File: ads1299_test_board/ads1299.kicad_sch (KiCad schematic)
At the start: 30 parts, among them U1 ADS1299, U4 OPA376xxD

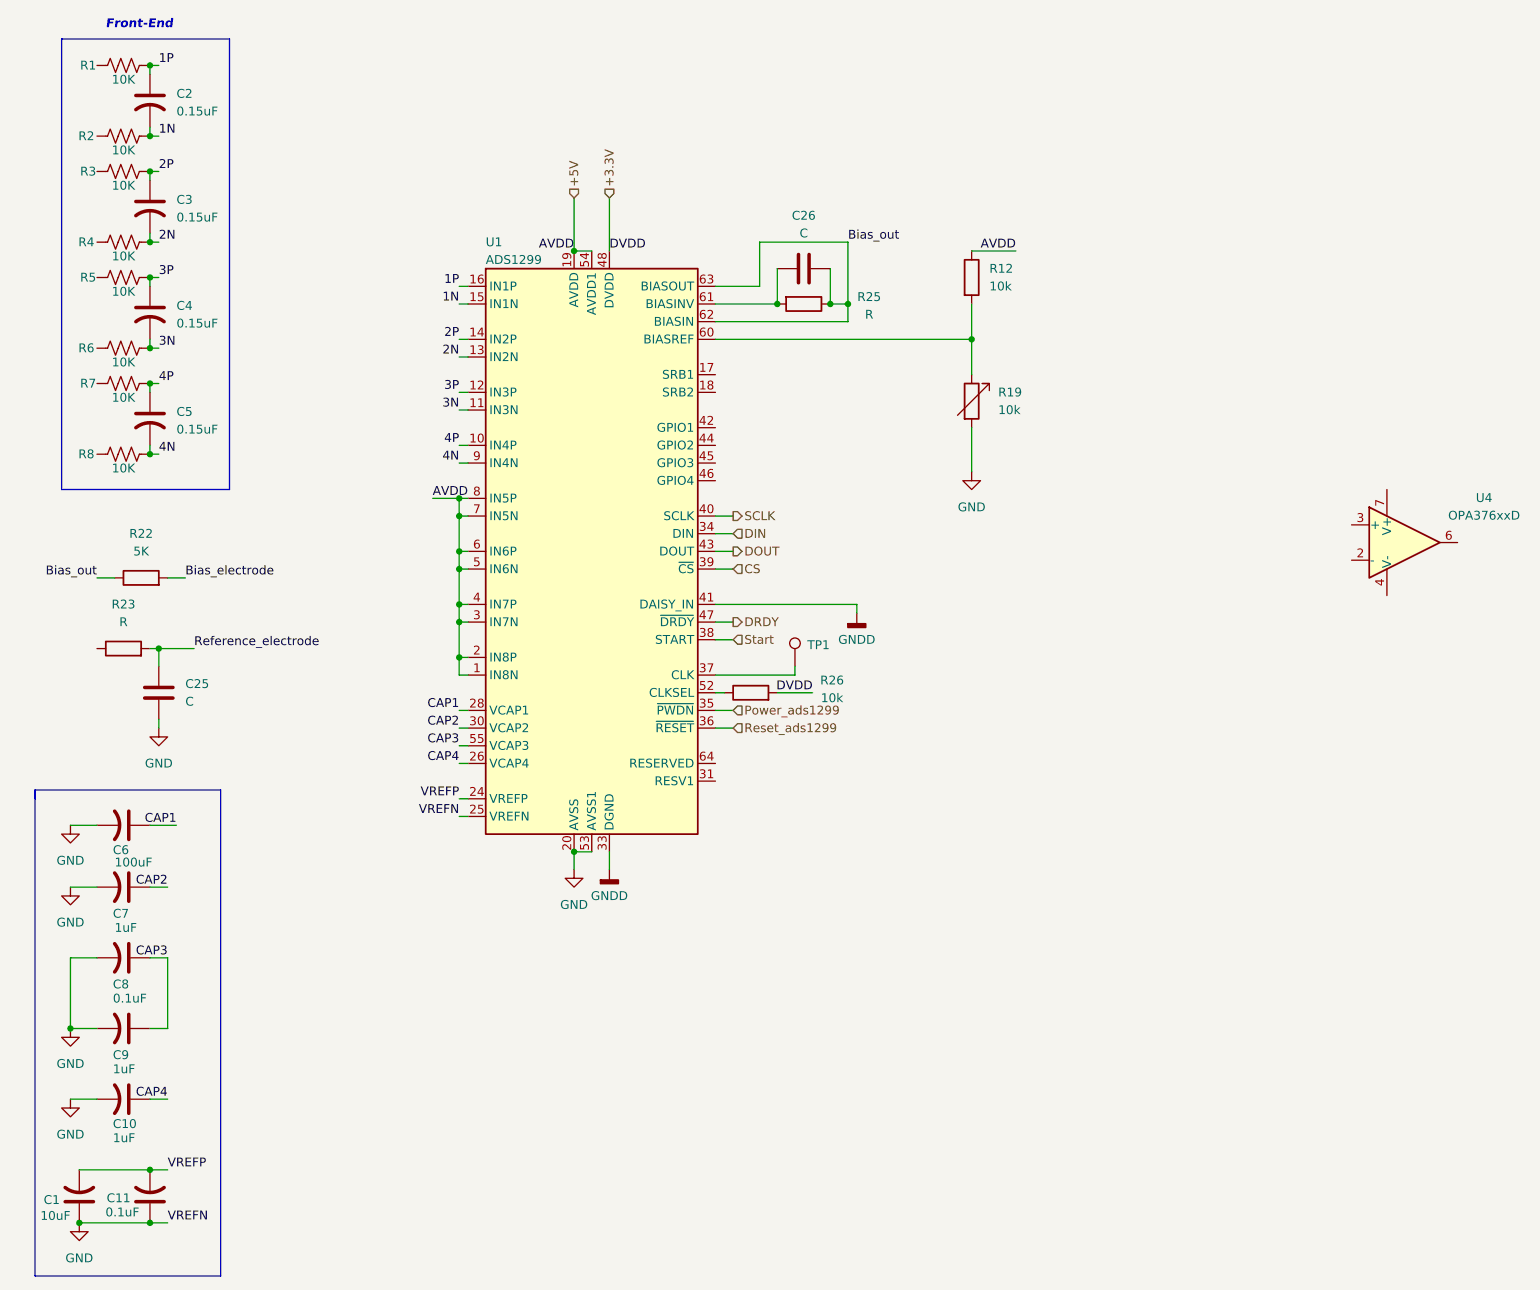
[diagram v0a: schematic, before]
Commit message: GPIO, SRB
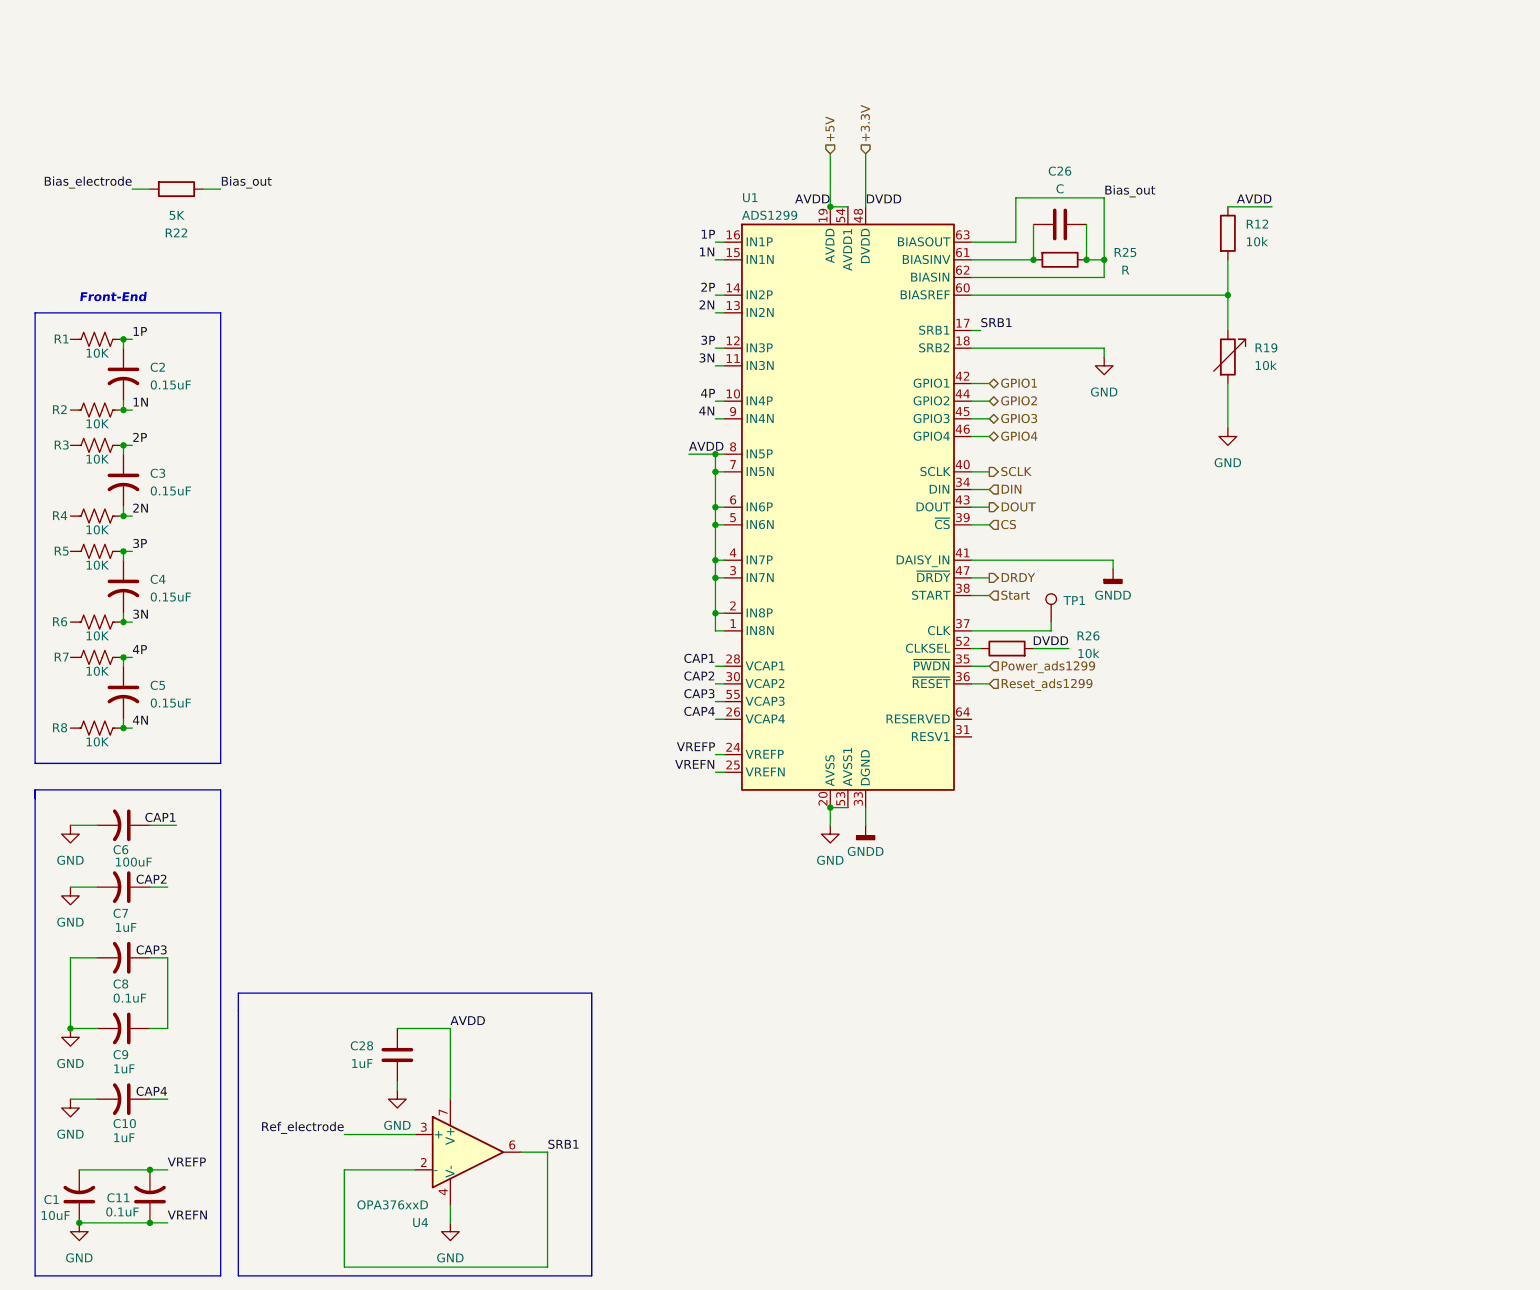
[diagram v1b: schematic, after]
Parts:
- removed C25: C, symbol Device:C
- removed R23: R, symbol Device:R
- added C28: 1uF, symbol Device:C
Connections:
- net +5V: now also U4.7 (V+), C28.1
- net GND: now also U1.18 (SRB2), U4.4 (V-), C28.2
- net SRB1: now reaches U1.17 (SRB1)
- net SRB1: now also U4.2 (-), U4.6
- net GPIO1: now reaches U1.42 (GPIO1)
- net GPIO2: now reaches U1.44 (GPIO2)
- net GPIO3: now reaches U1.45 (GPIO3)
- net GPIO4: now reaches U1.46 (GPIO4)
- net Ref_electrode: now reaches U4.3 (+)
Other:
- moved on the sheet: C2, C26, C3, C4, C5, R1, R12, R19, R2, R22, R25, R26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

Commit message: updates
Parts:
- C1, C10, C11, C28, C7, C8, C9, R22: footprint (none) -> Capacitor_SMD:C_0402_1005Metric_Pad0.74x0.62mm_HandSolder
- C2, C3, C4, C5: footprint (none) -> Capacitor_SMD:C_0603_1608Metric_Pad1.08x0.95mm_HandSolder
- C6: footprint (none) -> Capacitor_SMD:C_1206_3216Metric_Pad1.33x1.80mm_HandSolder
- R1, R12, R19, R2, R26, R3, R4, R5, R6, R7, R8: footprint (none) -> Resistor_SMD:R_0402_1005Metric_Pad0.72x0.64mm_HandSolder
- TP1: footprint (none) -> TestPoint:TestPoint_Pad_D1.5mm
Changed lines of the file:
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@@
 			)
 		)
-		(property "Footprint" ""
+		(property "Footprint" "Capacitor_SMD:C_0402_1005Metric_Pad0.74x0.62mm_HandSolder"
 			(at 29.21 149.86 0)
 			(hide yes)
@@
 			)
 		)
-		(property "Footprint" ""
+		(property "Footprint" "Capacitor_SMD:C_0402_1005Metric_Pad0.74x0.62mm_HandSolder"
 			(at 29.21 160.02 0)
 			(hide yes)
@@
 			)
 		)
-		(property "Footprint" ""
+		(property "Footprint" "Capacitor_SMD:C_0402_1005Metric_Pad0.74x0.62mm_HandSolder"
 			(at 29.21 170.18 0)
 			(hide yes)
@@
 			)
 		)
-		(property "Footprint" ""
+		(property "Footprint" "Capacitor_SMD:C_0402_1005Metric_Pad0.74x0.62mm_HandSolder"
 			(at 33.02 184.15 0)
 			(hide yes)
@@
 			)
 		)
-		(property "Footprint" ""
+		(property "Footprint" "Resistor_SMD:R_0402_1005Metric_Pad0.72x0.64mm_HandSolder"
 			(at 186.182 45.72 90)
 			(hide yes)
@@
 			)
 		)
-		(property "Footprint" ""
+		(property "Footprint" "Resistor_SMD:R_0402_1005Metric_Pad0.72x0.64mm_HandSolder"
 			(at 156.21 107.188 90)
 			(hide yes)
@@
 			)
 		)
-		(property "Footprint" ""
+		(property "Footprint" "Capacitor_SMD:C_0402_1005Metric_Pad0.74x0.62mm_HandSolder"
 			(at 22.86 184.15 0)
 			(hide yes)
@@
 			)
 		)
-		(property "Footprint" ""
+		(property "Footprint" "Resistor_SMD:R_0402_1005Metric_Pad0.72x0.64mm_HandSolder"
 			(at 25.654 85.344 90)
 			(hide yes)
@@
 			)
 		)
-		(property "Footprint" ""
+		(property "Footprint" "Resistor_SMD:R_0402_1005Metric_Pad0.72x0.64mm_HandSolder"
 			(at 25.654 75.184 90)
 			(hide yes)
@@
 			)
 		)
-		(property "Footprint" ""
+		(property "Footprint" "Capacitor_SMD:C_0603_1608Metric_Pad1.08x0.95mm_HandSolder"
 			(at 29.21 81.28 0)
 			(hide yes)
@@
 			)
 		)
-		(property "Footprint" ""
+		(property "Footprint" "Resistor_SMD:R_0402_1005Metric_Pad0.72x0.64mm_HandSolder"
 			(at 25.654 115.824 90)
 			(hide yes)
@@
 			)
 		)
-		(property "Footprint" ""
+		(property "Footprint" "Resistor_SMD:R_0402_1005Metric_Pad0.72x0.64mm_HandSolder"
 			(at 25.654 70.104 90)
 			(hide yes)
@@
 			)
 		)
-		(property "Footprint" ""
+		(property "Footprint" "Resistor_SMD:R_0402_1005Metric_Pad0.72x0.64mm_HandSolder"
 			(at 25.654 90.424 90)
 			(hide yes)
@@
 			)
 		)
-		(property "Footprint" ""
+		(property "Footprint" "Capacitor_SMD:C_0402_1005Metric_Pad0.74x0.62mm_HandSolder"
 			(at 36.83 37.592 90)
 			(hide yes)
@@
 			)
 		)
-		(property "Footprint" ""
+		(property "Footprint" "Resistor_SMD:R_0402_1005Metric_Pad0.72x0.64mm_HandSolder"
 			(at 186.182 63.5 90)
 			(hide yes)
@@
 			)
 		)
-		(property "Footprint" ""
+		(property "Footprint" "Capacitor_SMD:C_0603_1608Metric_Pad1.08x0.95mm_HandSolder"
 			(at 29.21 96.52 0)
 			(hide yes)
@@
 			)
 		)
-		(property "Footprint" ""
+		(property "Footprint" "Resistor_SMD:R_0402_1005Metric_Pad0.72x0.64mm_HandSolder"
 			(at 25.654 105.664 90)
 			(hide yes)
@@
 			)
 		)
-		(property "Footprint" ""
+		(property "Footprint" "Capacitor_SMD:C_1206_3216Metric_Pad1.33x1.80mm_HandSolder"
 			(at 29.21 130.81 0)
 			(hide yes)
@@
 			)
 		)
-		(property "Footprint" ""
+		(property "Footprint" "TestPoint:TestPoint_Pad_D1.5mm"
 			(at 167.64 101.6 0)
 			(hide yes)
@@
 			)
 		)
-		(property "Footprint" ""
+		(property "Footprint" "Resistor_SMD:R_0402_1005Metric_Pad0.72x0.64mm_HandSolder"
 			(at 25.654 59.944 90)
 			(hide yes)
@@
 			)
 		)
-		(property "Footprint" ""
+		(property "Footprint" "Capacitor_SMD:C_0402_1005Metric_Pad0.74x0.62mm_HandSolder"
 			(at 69.5452 167.64 0)
 			(hide yes)
@@
 			)
 		)
-		(property "Footprint" ""
+		(property "Footprint" "Capacitor_SMD:C_0402_1005Metric_Pad0.74x0.62mm_HandSolder"
 			(at 29.21 139.7 0)
 			(hide yes)
@@
 			)
 		)
-		(property "Footprint" ""
+		(property "Footprint" "Capacitor_SMD:C_0603_1608Metric_Pad1.08x0.95mm_HandSolder"
 			(at 29.21 111.76 0)
 			(hide yes)
@@
 			)
 		)
-		(property "Footprint" ""
+		(property "Footprint" "Capacitor_SMD:C_0603_1608Metric_Pad1.08x0.95mm_HandSolder"
 			(at 29.21 66.04 0)
 			(hide yes)
@@
 			)
 		)
-		(property "Footprint" ""
+		(property "Footprint" "Resistor_SMD:R_0402_1005Metric_Pad0.72x0.64mm_HandSolder"
 			(at 25.654 100.584 90)
 			(hide yes)
